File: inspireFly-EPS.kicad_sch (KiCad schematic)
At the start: 24 parts, among them J1 USB4085-GF-A_REVB, Q3 NMOS, Q4 NMOS, U1 STM32U575RIT6, U2 BQ25750RRVR, U3 TCAN332DCNR

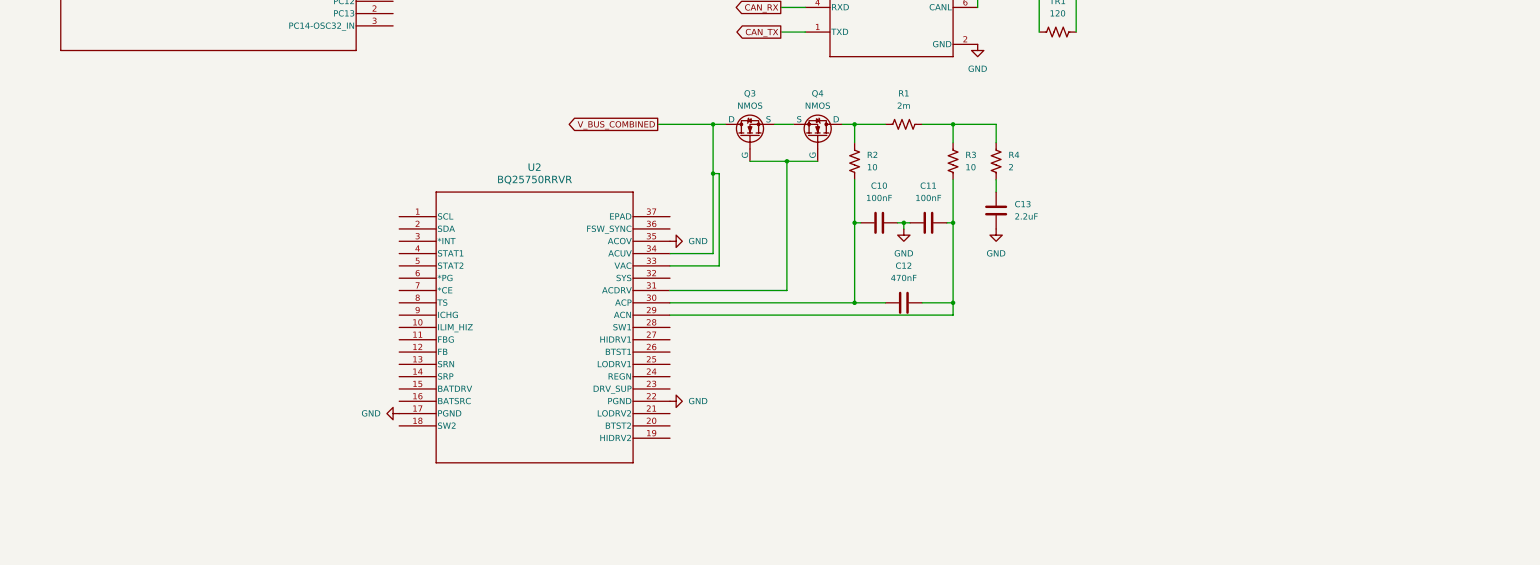
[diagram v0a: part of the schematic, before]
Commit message: Good progress on BQ chip - need to do math later
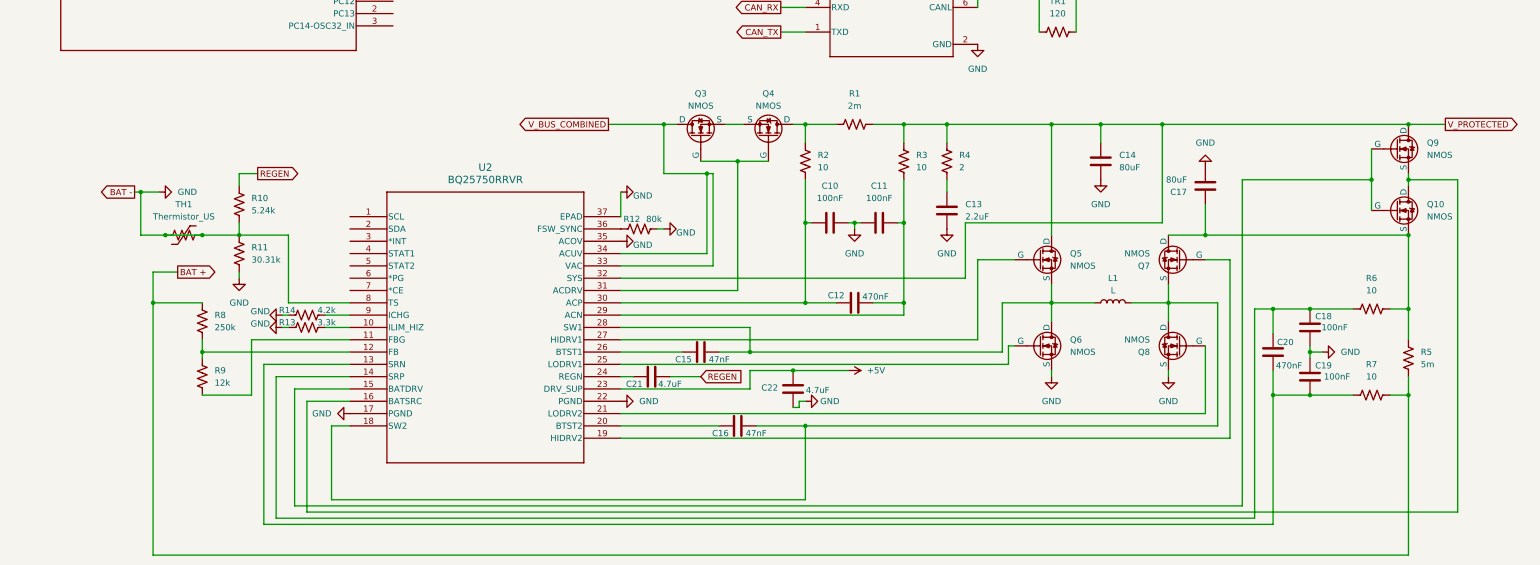
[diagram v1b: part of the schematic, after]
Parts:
- added C14, C17: 80uF, symbol Device:C
- added C15, C16: 47nF, symbol Device:C
- added C18, C19: 100nF, symbol Device:C
- added C20: 470nF, symbol Device:C
- added C21, C22: 4.7uF, symbol Device:C
- added L1: L, symbol Device:L
- added Q10, Q5, Q6, Q7, Q8, Q9: NMOS, symbol Simulation_SPICE:NMOS
- added R10: 5.24k, symbol Device:R_US
- added R11: 30.31k, symbol Device:R_US
- added R12: 80k, symbol Device:R_US
- added R13: 3.3k, symbol Device:R_US
- added R14: 4.2k, symbol Device:R_US
- added R5: 5m, symbol Device:R_US
- added R6, R7: 10, symbol Device:R_US
- added R8: 250k, symbol Device:R_US
- added R9: 12k, symbol Device:R_US
- added TH1: Thermistor_US, symbol Device:Thermistor_US
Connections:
- net GND: now also U2.37 (EPAD), U2.8 (TS), C14.2, C17.2, C18.2, C19.1, C22.1, Q6.3 (S), Q8.3 (S), R10.2, R11.1, R11.2, R12.2, R13.1, R14.1, TH1.1, TH1.2
- net V_PROTECTED: now reaches R1.2, R3.1, R4.1
- net V_PROTECTED: now also U2.32 (SYS), C14.1, Q5.1 (D), Q9.1 (D)
- net at U2.10 (ILIM_HIZ): now also R13.2
- net at U2.11 (FBG): now also R9.2
- net at U2.12 (FB): now also R8.2, R9.1
- net at U2.13 (SRN): now also C19.2, C20.1, R7.1
- net at U2.14 (SRP): now also C18.1, C20.2, R6.1
- net at U2.15 (BATDRV): now also Q10.2 (G), Q9.2 (G)
- net at U2.16 (BATSRC): now also Q10.1 (D), Q9.3 (S)
- net at U2.18 (SW2): now also C16.2, L1.2, Q7.3 (S), Q8.1 (D)
- net at U2.19 (HIDRV2): now also Q7.2 (G)
- net at U2.20 (BTST2): now also C16.1
- net at U2.21 (LODRV2): now also Q8.2 (G)
- net +5V: now reaches U2.23 (DRV_SUP)
- net +5V: now also C22.2
- net at U2.24 (REGN): now also C21.1
- net at U2.25 (LODRV1): now also Q6.2 (G)
- net at U2.26 (BTST1): now also C15.1
- net at U2.27 (HIDRV1): now also Q5.2 (G)
- net at U2.28 (SW1): now also C15.2, L1.1, Q5.3 (S), Q6.1 (D)
- net at U2.36 (FSW_SYNC): now also R12.1
- net at U2.9 (ICHG): now also R14.2
- new net: C17.1, Q10.3 (S), Q7.1 (D), R5.1, R6.2
- new net BAT +: R5.2, R7.2, R8.1
- new net REGEN: C21.2, R10.1
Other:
- moved on the sheet: C10, C11, C12, C13, Q3, Q4, R1, R2, R3, R4, U2
